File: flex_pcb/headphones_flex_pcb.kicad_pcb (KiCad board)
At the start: 2 copper layers, 42 x 25.2 mm, 15 parts, among them J1 LIGHTING_JACK, J2 CONN_01X01, J3 BOTTOM_FLEX_LIGHTNING, J5 LIGHTNING_HEADPHONE_ADAPTER, J7 IPHONE_HEADPHONE_JACK, U1 SN74LVC1G123, U2 SN74LVC1G123, U3 NC7S32-micropak6, U4 ADG774A-LFCSP

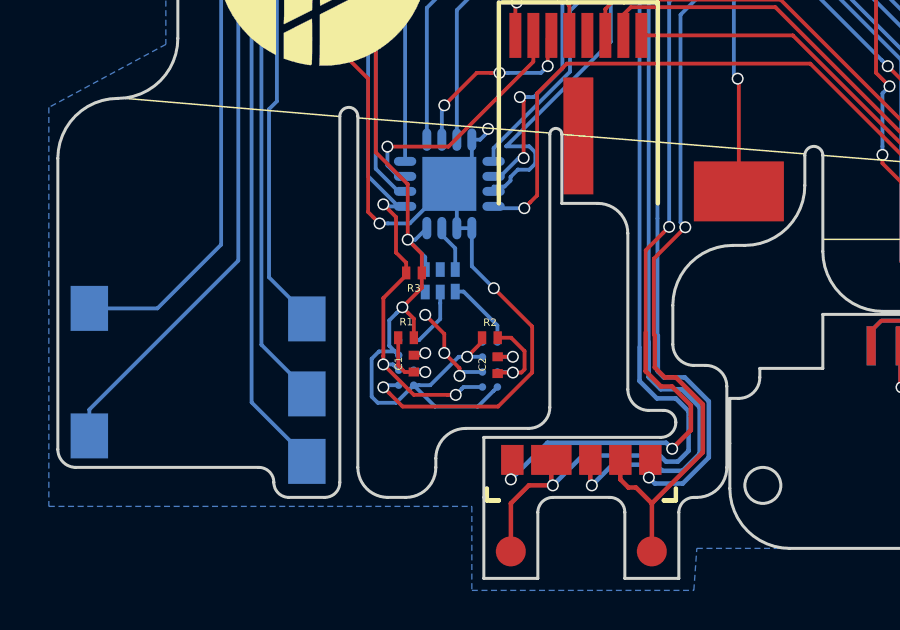
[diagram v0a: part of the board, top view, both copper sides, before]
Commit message: First flex pcb version - ready to fab. v0.9
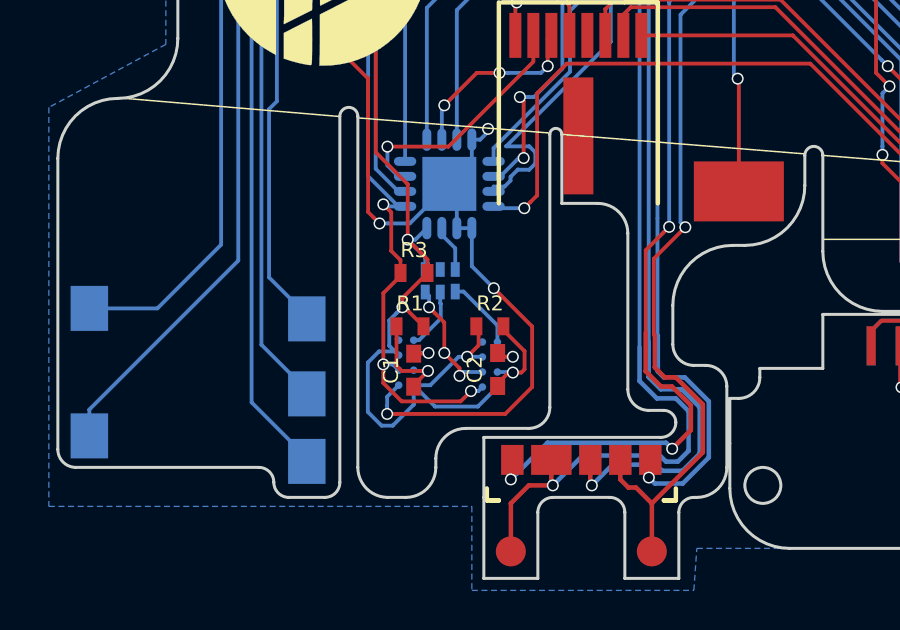
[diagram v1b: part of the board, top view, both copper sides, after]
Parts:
- C1, C2: footprint Capacitors_SMD:C_0201_NoSilk -> Capacitors_SMD:C_0402_NoSilk
- R1, R2, R3: footprint Resistors_SMD:R_0201_NoSilk -> Resistors_SMD:R_0402_NoSilk
- moved R1 0.40 mm to (134.2, 77.6)
- moved R2 0.38 mm to (136.9, 77.6)
- moved C1 0.22 mm to (134.4, 79.1)
- moved C2 0.14 mm to (137.2, 79.0)
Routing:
- net VCC: track 49.9 -> 51.7 mm
- net Net-(C1-Pad1): track 2.33 -> 3.73 mm
- net GNDREF: track 50.9 -> 52.3 mm
